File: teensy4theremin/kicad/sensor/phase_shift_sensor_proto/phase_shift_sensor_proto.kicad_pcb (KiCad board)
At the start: 2 copper layers, 24 parts, among them J1 SENSOR, J2 L_IN, J3 L_OUT, J4 ANT, Q1 2N3904, U1 74HC04, U2 sp721, U3 REG_3V3

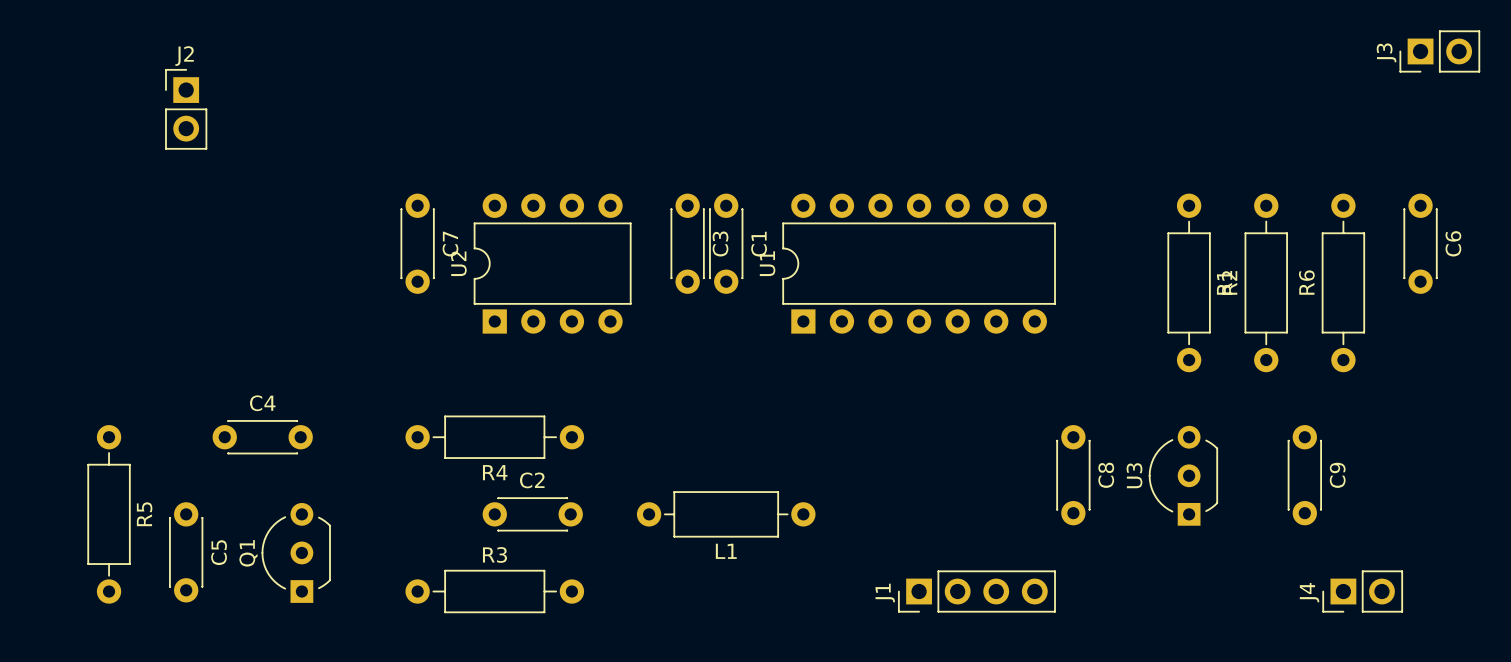
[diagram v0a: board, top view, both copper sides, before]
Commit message: phase shift sensor PCB
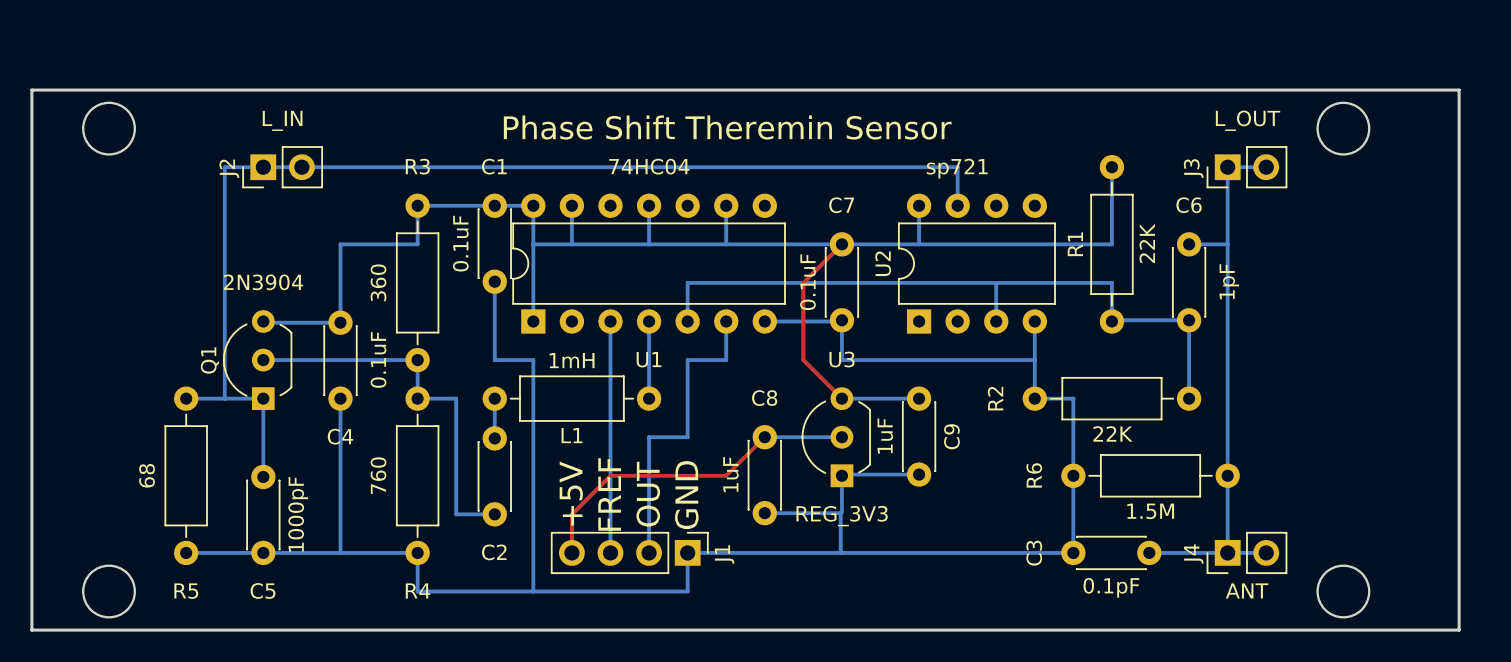
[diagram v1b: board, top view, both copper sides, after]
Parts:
- C3: value 10uF -> 0.1pF
- moved C3 34.2 mm to (129.5, 116.8), turned to 0 degrees
- moved C7 28.1 mm to (114.3, 96.5)
- moved U2 27.9 mm to (119.4, 101.6)
- moved C9 25.5 mm to (119.4, 106.7)
- moved U3 23.0 mm to (114.3, 111.8)
- moved C8 20.3 mm to (109.2, 109.2)
- moved R6 19.3 mm to (129.5, 111.8), turned to 0 degrees
- moved U1 17.8 mm to (94.0, 101.6)
- moved R2 15.5 mm to (127.0, 106.7), turned to 0 degrees
- moved C6 15.5 mm to (137.2, 96.5)
- moved J1 15.5 mm to (104.1, 116.8), turned to 270 degrees
- moved C1 15.2 mm to (91.4, 94.0)
- moved R3 15.2 mm to (86.4, 104.1), turned to 90 degrees
- moved J3 14.8 mm to (139.7, 91.4)
- moved Q1 13.0 mm to (76.2, 106.7)
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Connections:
- C3 pad 1: +3V3 -> GND
- C3 pad 2: GND -> Net-(C3-Pad2)
- C6 pad 1: Net-(C6-Pad1) -> Net-(C3-Pad2)
- J3 pad 1: Net-(C6-Pad1) -> Net-(C3-Pad2)
- J3 pad 2: Net-(C6-Pad1) -> Net-(C3-Pad2)
- J4 pad 1: Net-(C6-Pad1) -> Net-(C3-Pad2)
- J4 pad 2: Net-(C6-Pad1) -> Net-(C3-Pad2)
- R6 pad 2: Net-(C6-Pad1) -> Net-(C3-Pad2)
- U1 pad 1: /REF_CLK -> +3V3
- U1 pad 2: Net-(L1-Pad1) -> Net-(U1-Pad2)
- U1 pad 3: Net-(C6-Pad2) -> /REF_CLK
- U1 pad 4: /PWM_OUT -> Net-(L1-Pad1)
- U1 pad 5: +3V3 -> Net-(C6-Pad2)
- U1 pad 6: Net-(U1-Pad6) -> /PWM_OUT
- U2 pad 1: Net-(C6-Pad2) -> Net-(U2-Pad1)
- U2 pad 3: Net-(U2-Pad3) -> Net-(C6-Pad2)
- U2 pad 5: Net-(C5-Pad2) -> Net-(U2-Pad5)
- U2 pad 7: Net-(U2-Pad7) -> Net-(C5-Pad2)
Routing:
- net GND: track 0.00 -> 150.1 mm
- net +3V3: track 0.00 -> 103.8 mm
- net Net-(C5-Pad2): track 0.00 -> 76.3 mm
- net Net-(C6-Pad2): track 0.00 -> 45.8 mm
- net Net-(C3-Pad2): track 0.00 -> 38.2 mm
- net Net-(C2-Pad1): track 0.00 -> 25.4 mm
- net +5V: track 0.00 -> 22.4 mm
- net /PWM_OUT: track 0.00 -> 20.3 mm
- net /REF_CLK: track 0.00 -> 15.2 mm
- net Net-(L1-Pad1): track 0.00 -> 5.08 mm
- net Net-(C2-Pad2): track 0.00 -> 2.62 mm
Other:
- board outline added: 94 x 35.6 mm
- board text added: "+5V"
- board text added: "FREF"
- board text added: "GND"
- board text added: "OUT"
- board text added: "Phase Shift Theremin Sensor"
